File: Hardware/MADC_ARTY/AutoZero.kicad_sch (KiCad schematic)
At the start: 8 parts, among them U11 ADG419BRM, U12 ADG419BRM, U13 ADG419BRM, U14 ADG419BRM

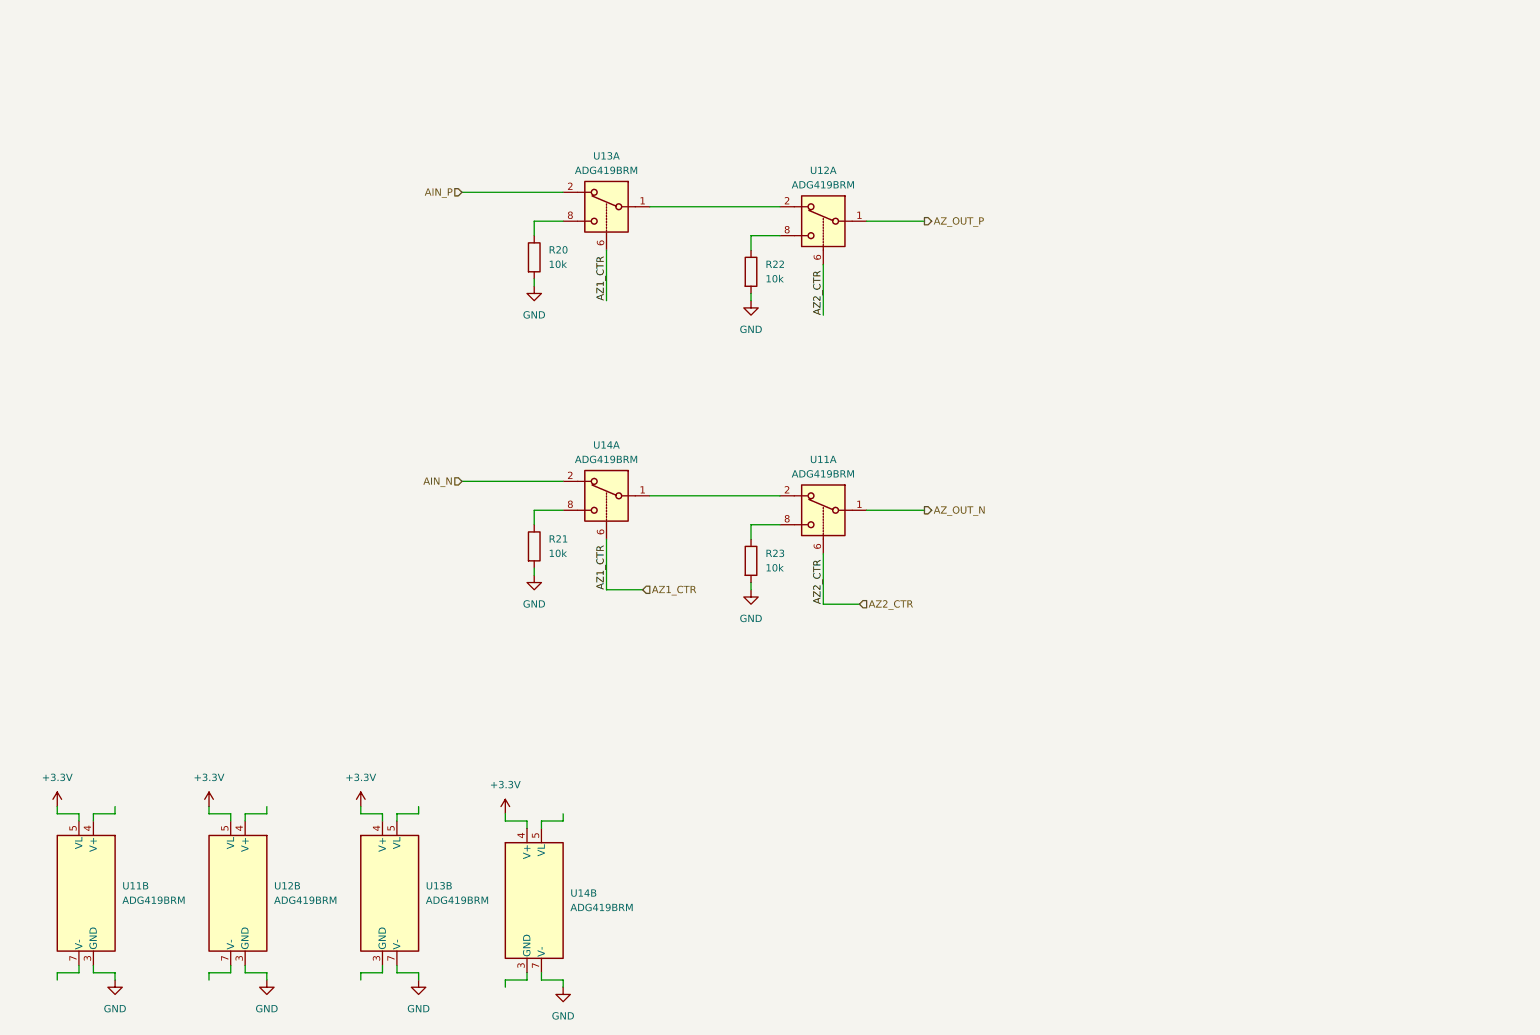
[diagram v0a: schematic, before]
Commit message: Schematic
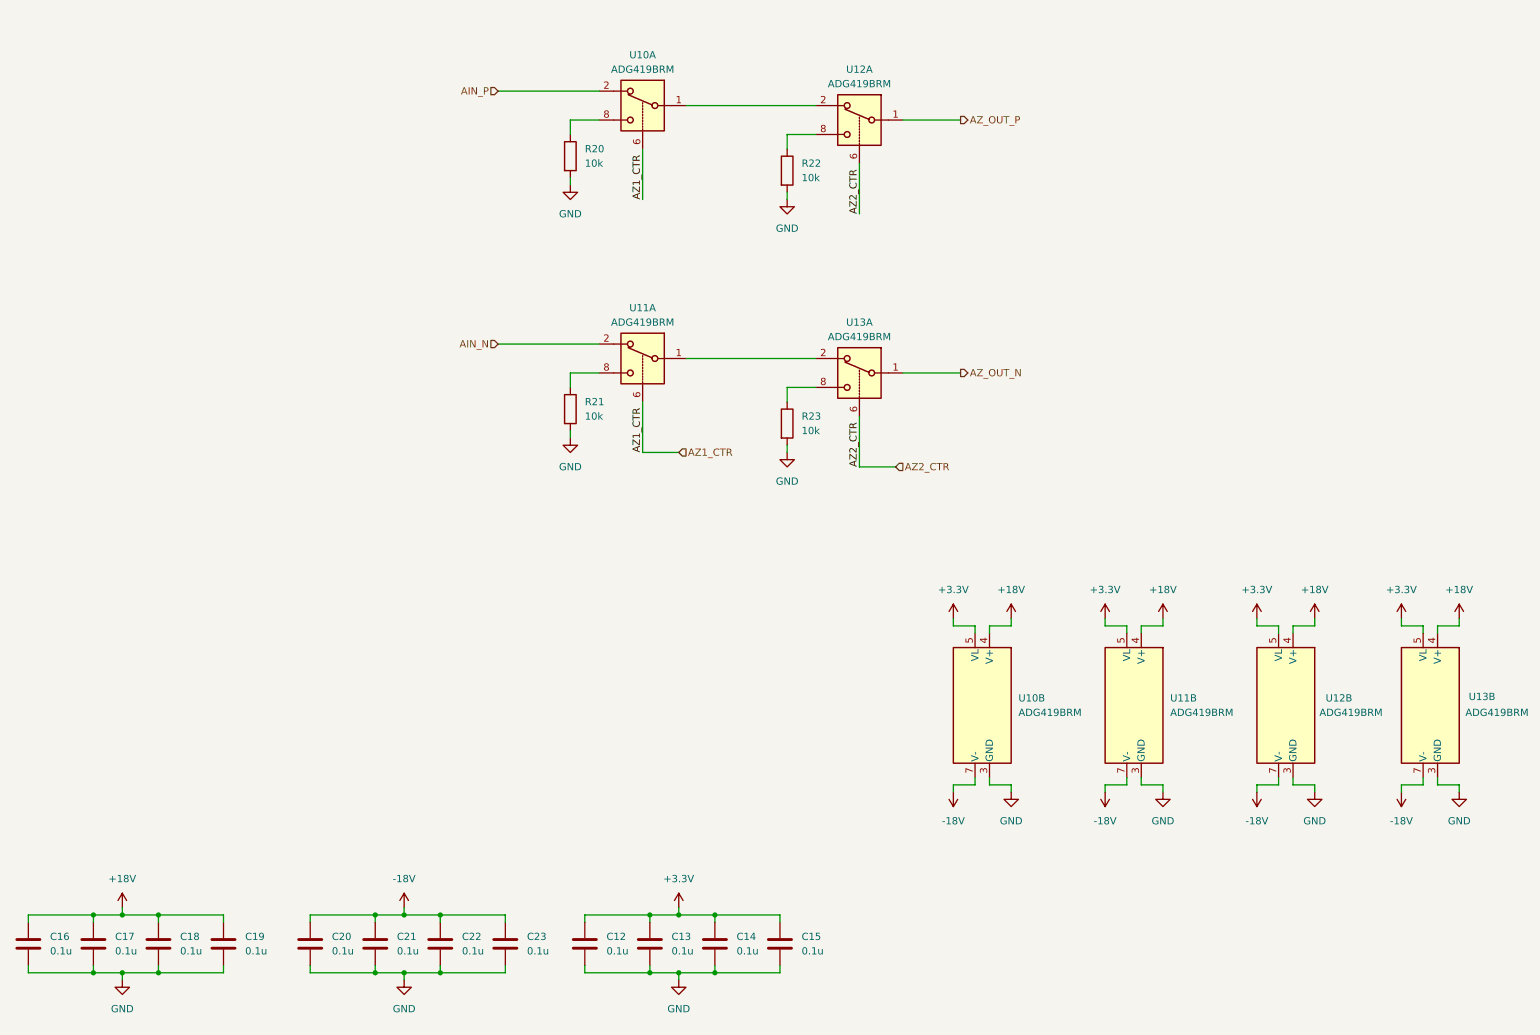
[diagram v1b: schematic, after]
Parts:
- added C12, C13, C14, C15, C16, C17, C18, C19, C20, C21, C22, C23: 0.1u, symbol Device:C
- renumbered U13 to U10, U11 to U10, U14 to U11, U12 to U11, U13 to U12, U11 to U13, U14 to U13
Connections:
- net +3.3V: now also U12.5 (VL), U13.5 (VL), C12.1, C13.1, C14.1, C15.1; no longer U12.4 (V+), U13.4 (V+)
- net GND: now also U12.3 (GND), U13.3 (GND), C12.2, C13.2, C14.2, C15.2, C16.2, C17.2, C18.2, C19.2, C20.2, C21.2, C22.2, C23.2; no longer U12.7 (V-), U13.7 (V-)
- net +18V: now reaches U10.4 (V+)
- net +18V: now also U11.4 (V+), U12.4 (V+), U13.4 (V+), C16.1, C17.1, C18.1, C19.1
- net -18V: now reaches U10.7 (V-)
- net -18V: now also U11.7 (V-), U12.7 (V-), U13.7 (V-), C20.1, C21.1, C22.1, C23.1
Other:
- moved on the sheet: R20, R21, R22, R23, U10A, U10B, U11A, U11B, U12A, U12B, U13A, U13B

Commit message: Schematic
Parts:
- C12, C13, C14, C15, C16, C17, C18, C19, C20, C21, C22, C23: footprint (none) -> Capacitor_SMD:C_0603_1608Metric
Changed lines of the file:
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@@
 			)
 		)
-		(property "Footprint" ""
+		(property "Footprint" "Capacitor_SMD:C_0603_1608Metric"
 			(at 91.1352 186.69 0)
 			(effects
@@
 			)
 		)
-		(property "Footprint" ""
+		(property "Footprint" "Capacitor_SMD:C_0603_1608Metric"
 			(at 102.5652 186.69 0)
 			(effects
@@
 			)
 		)
-		(property "Footprint" ""
+		(property "Footprint" "Capacitor_SMD:C_0603_1608Metric"
 			(at 30.1752 186.69 0)
 			(effects
@@
 			)
 		)
-		(property "Footprint" ""
+		(property "Footprint" "Capacitor_SMD:C_0603_1608Metric"
 			(at 41.6052 186.69 0)
 			(effects
@@
 			)
 		)
-		(property "Footprint" ""
+		(property "Footprint" "Capacitor_SMD:C_0603_1608Metric"
 			(at 68.2752 186.69 0)
 			(effects
@@
 			)
 		)
-		(property "Footprint" ""
+		(property "Footprint" "Capacitor_SMD:C_0603_1608Metric"
 			(at 79.7052 186.69 0)
 			(effects
@@
 			)
 		)
-		(property "Footprint" ""
+		(property "Footprint" "Capacitor_SMD:C_0603_1608Metric"
 			(at 53.0352 186.69 0)
 			(effects
@@
 			)
 		)
-		(property "Footprint" ""
+		(property "Footprint" "Capacitor_SMD:C_0603_1608Metric"
 			(at 150.8252 186.69 0)
 			(effects
@@
 			)
 		)
-		(property "Footprint" ""
+		(property "Footprint" "Capacitor_SMD:C_0603_1608Metric"
 			(at 116.5352 186.69 0)
 			(effects
@@
 			)
 		)
-		(property "Footprint" ""
+		(property "Footprint" "Capacitor_SMD:C_0603_1608Metric"
 			(at 18.7452 186.69 0)
 			(effects
@@
 			)
 		)
-		(property "Footprint" ""
+		(property "Footprint" "Capacitor_SMD:C_0603_1608Metric"
 			(at 139.3952 186.69 0)
 			(effects
@@
 			)
 		)
-		(property "Footprint" ""
+		(property "Footprint" "Capacitor_SMD:C_0603_1608Metric"
 			(at 127.9652 186.69 0)
 			(effects

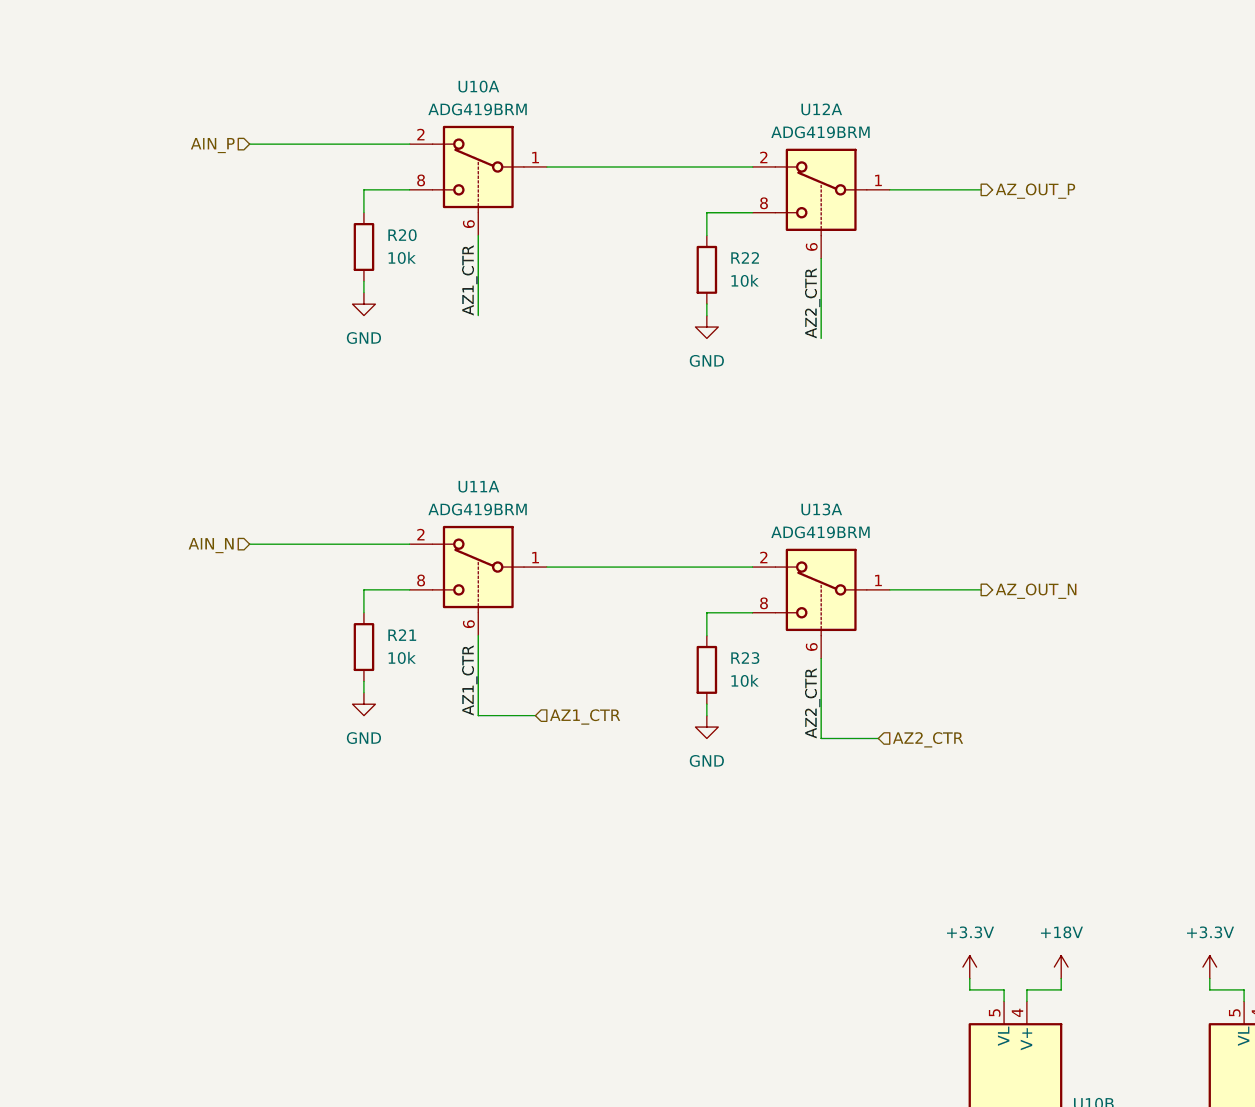
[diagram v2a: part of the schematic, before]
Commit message: Schematic
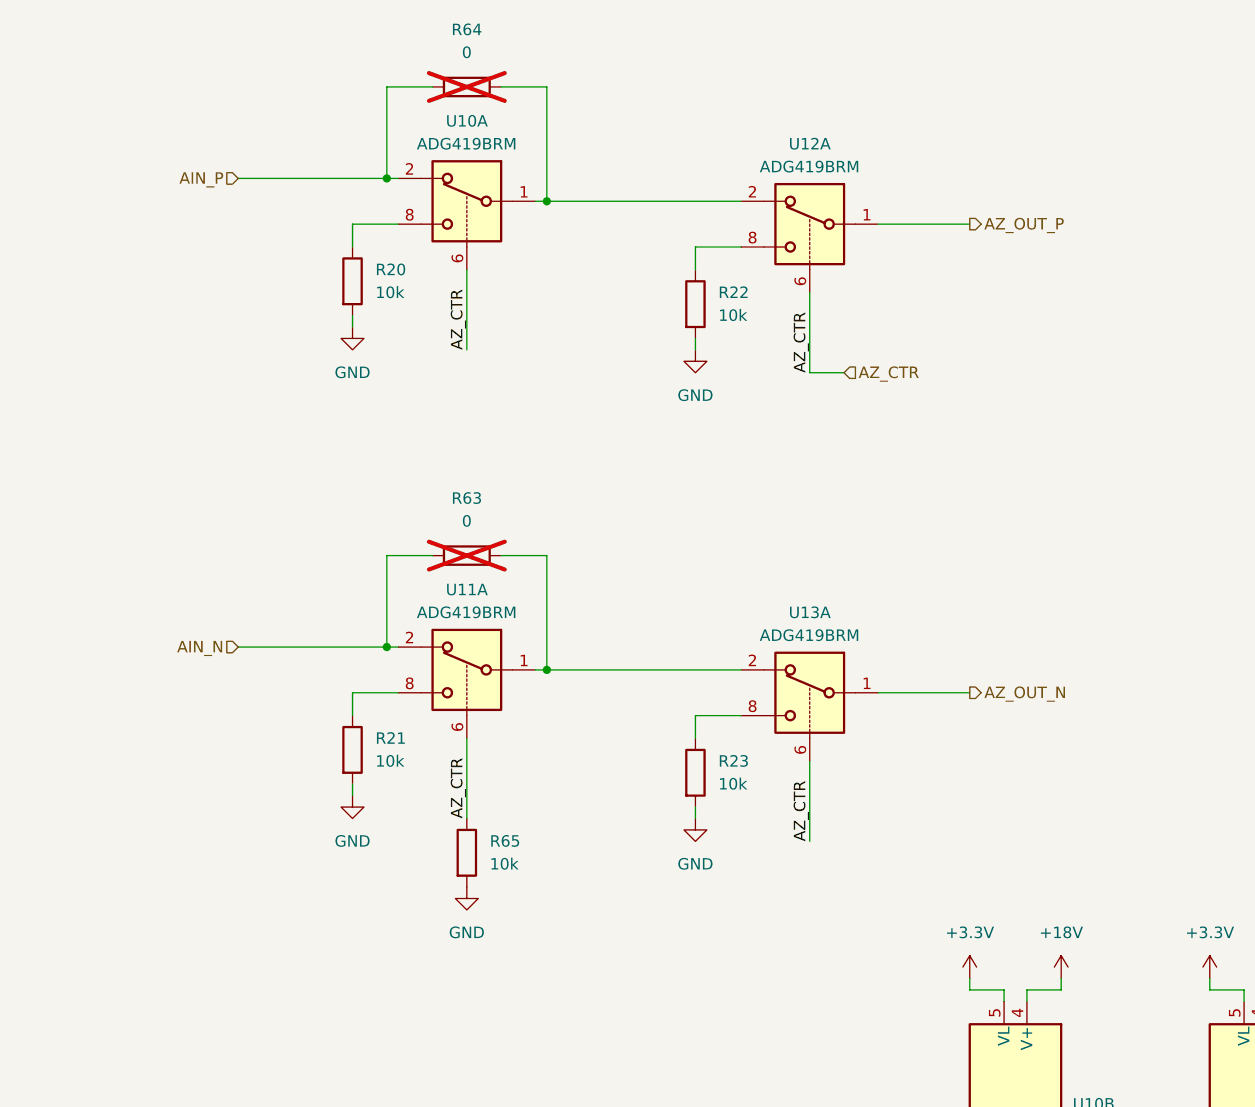
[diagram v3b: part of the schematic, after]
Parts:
- added R63, R64: 0, Resistor_SMD:R_0603_1608Metric, symbol Device:R
- added R65: 10k, Resistor_SMD:R_0603_1608Metric, symbol Device:R
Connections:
- net AZ2_CTR is gone; now on net AZ_CTR: U12.6, U13.6
- net AIN_N: now also R63.1
- net AIN_P: now also R64.1
- net GND: now also R65.2
- net at U10.1, U12.2: now also R64.2
- net at U11.1, U13.2: now also R63.2
- net AZ1_CTR renamed AZ_CTR
- net AZ_CTR: now also R65.1
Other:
- moved on the sheet: R20, R21, R22, R23, U10A, U11A, U12A, U13A

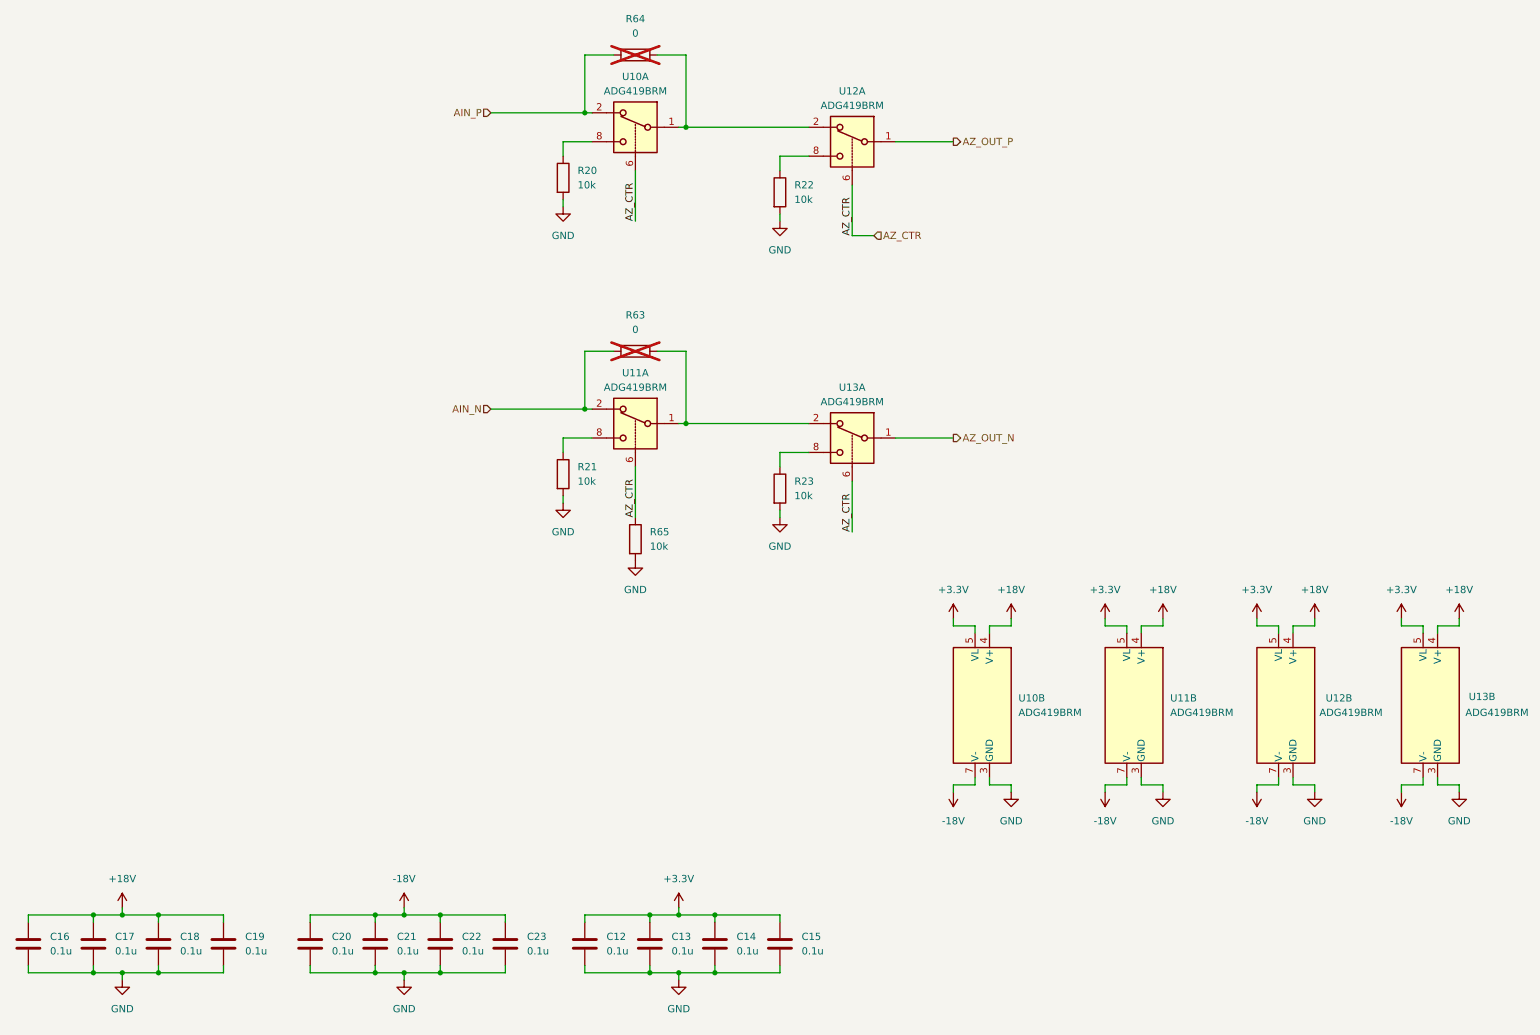
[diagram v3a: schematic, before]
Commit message: PCB and Schematic
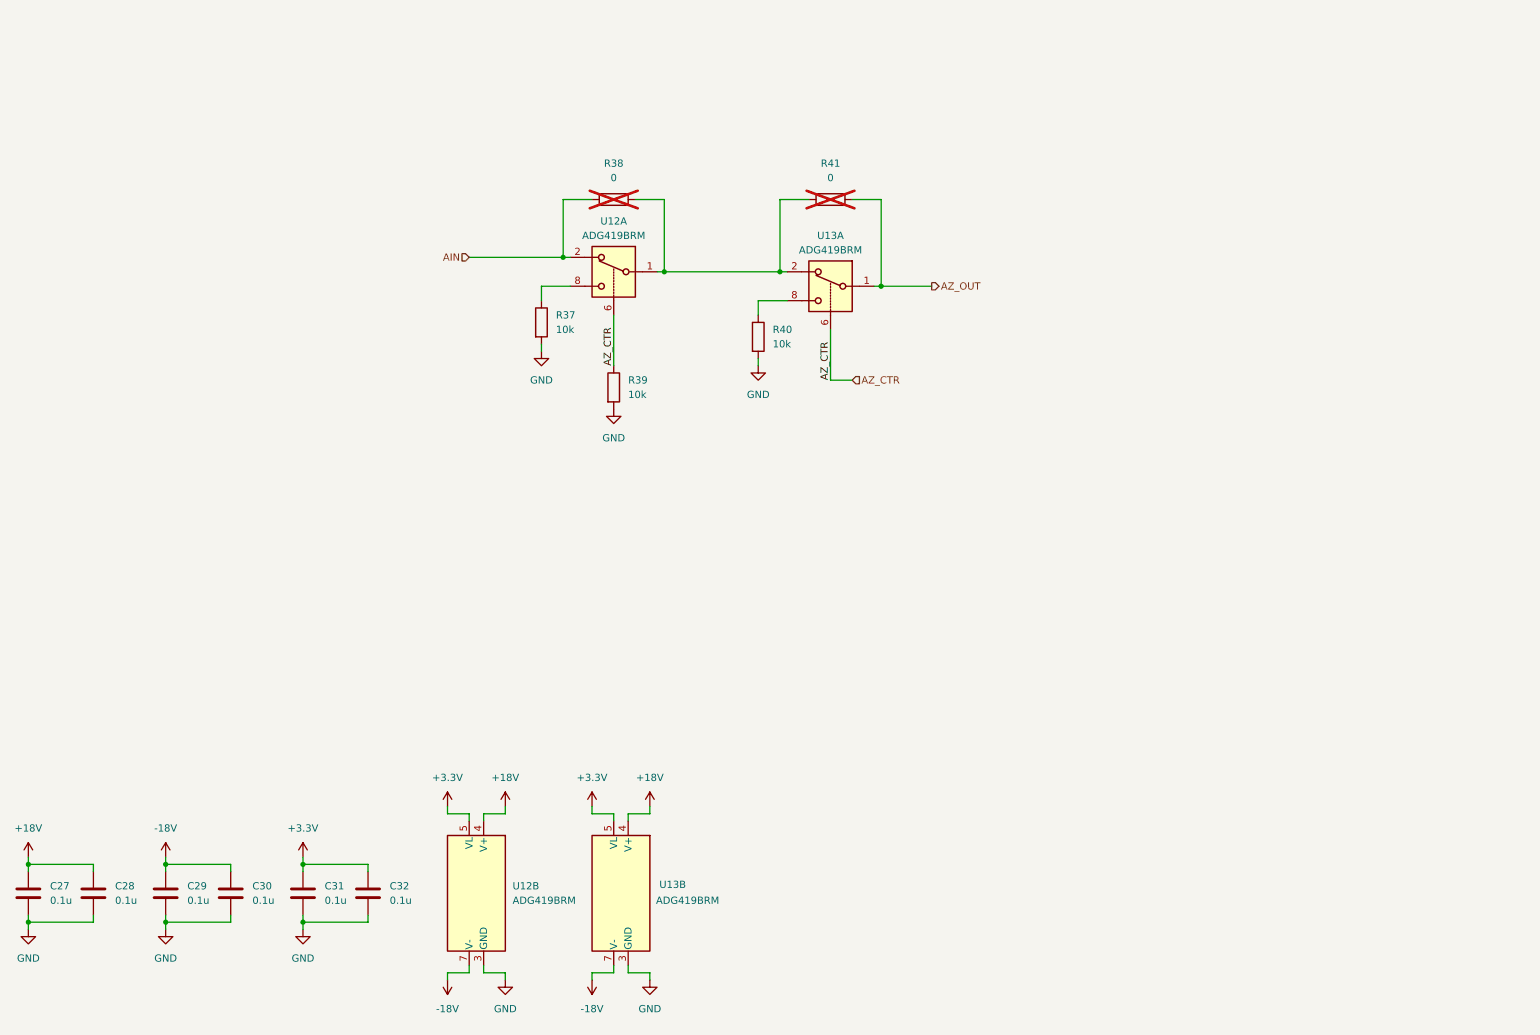
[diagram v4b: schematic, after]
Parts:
- removed C12, C13, C16, C17, C20, C21: 0.1u, Capacitor_SMD:C_0603_1608Metric, symbol Device:C
- removed R20, R22: 10k, Resistor_SMD:R_0603_1608Metric, symbol Device:R
- removed R64: 0, Resistor_SMD:R_0603_1608Metric, symbol Device:R
- removed U10, U12: ADG419BRM, Package_SO:MSOP-8_3x3mm_P0.65mm, symbol Analog_Switch:ADG419BRM
- added R41: 0, Resistor_SMD:R_0603_1608Metric, symbol Device:R
- renumbered C18 to C27, C19 to C28, C22 to C29, C23 to C30, C14 to C31, C15 to C32, R21 to R37, R63 to R38, R65 to R39, R23 to R40, U11 to U12
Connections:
- net at R38.2, U12.1, U13.2: now also R41.1
- net AIN_N renamed AIN
- net AZ_OUT_N renamed AZ_OUT
- net AZ_OUT: now also R41.2
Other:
- moved on the sheet: C27, C28, C29, C30, C31, C32, R37, R38, R39, R40, U12A, U12B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
